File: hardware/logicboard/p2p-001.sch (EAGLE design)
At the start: 28 parts, among them IC11 74ALS04N, J0 DC9V, J11 AUDIO_JACK_3.5MM_PTH, J12 AUDIO_JACK_3.5MM_PTH, J13 AUDIO_JACK_3.5MM_PTH, J14 AUDIO_JACK_3.5MM_PTH, J7 DIN5, J8 DIN5, J9 DIN5, X0 MKDSN1,5/2-5,08

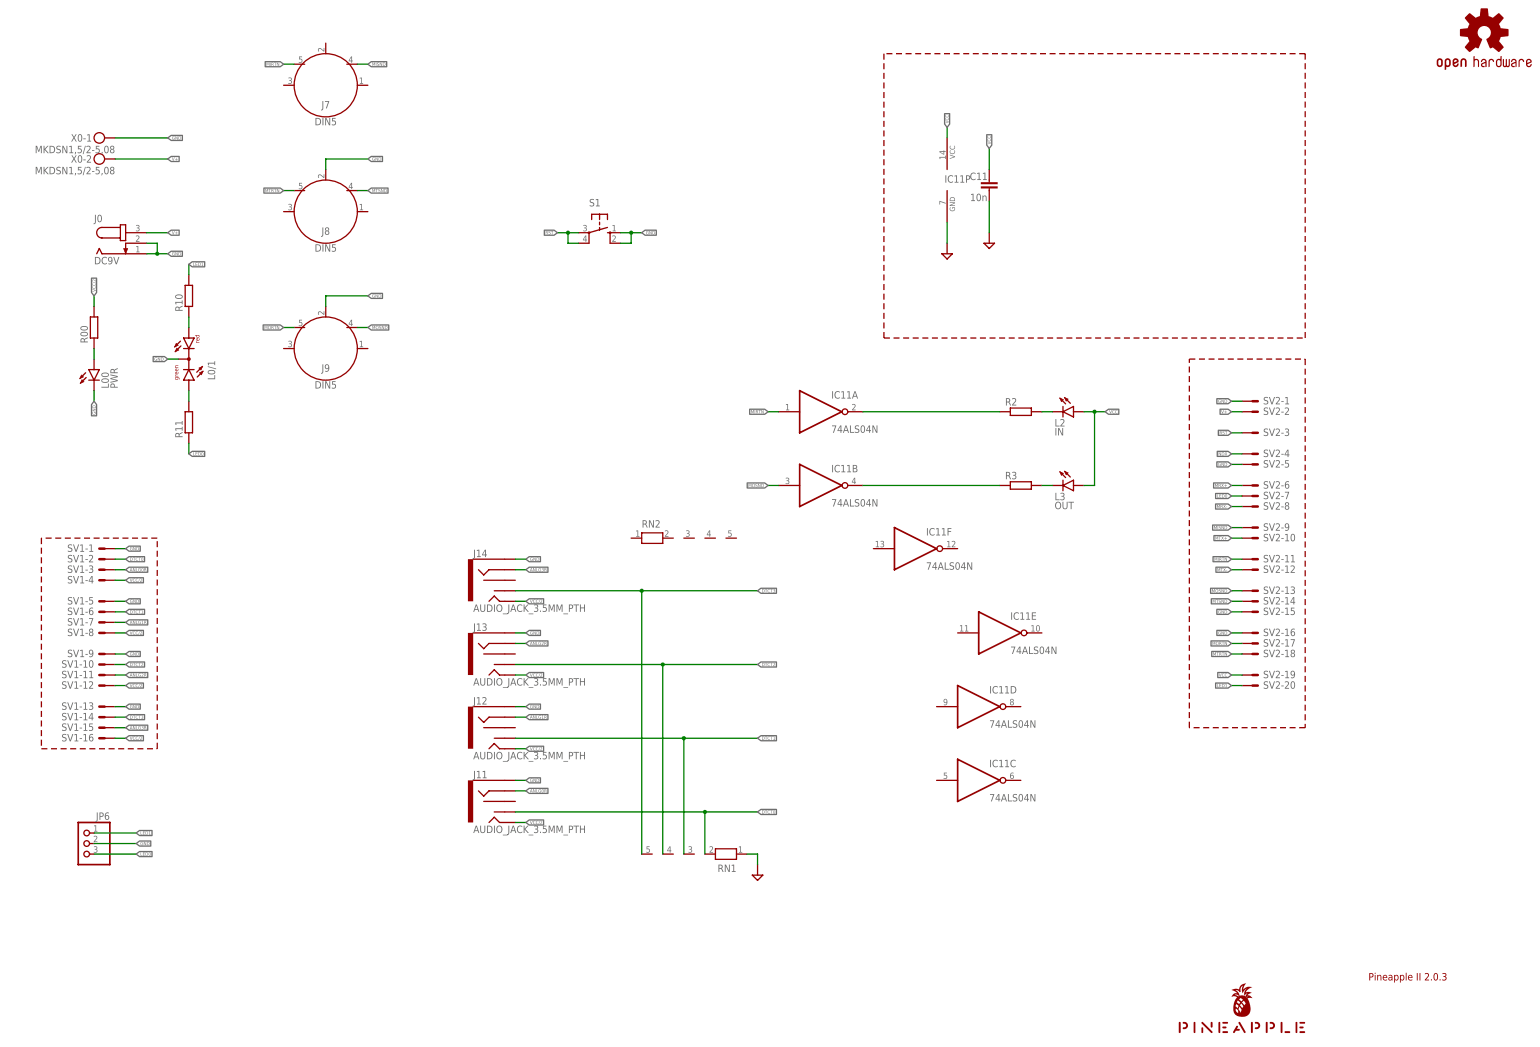
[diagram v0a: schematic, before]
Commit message: Cloud work...
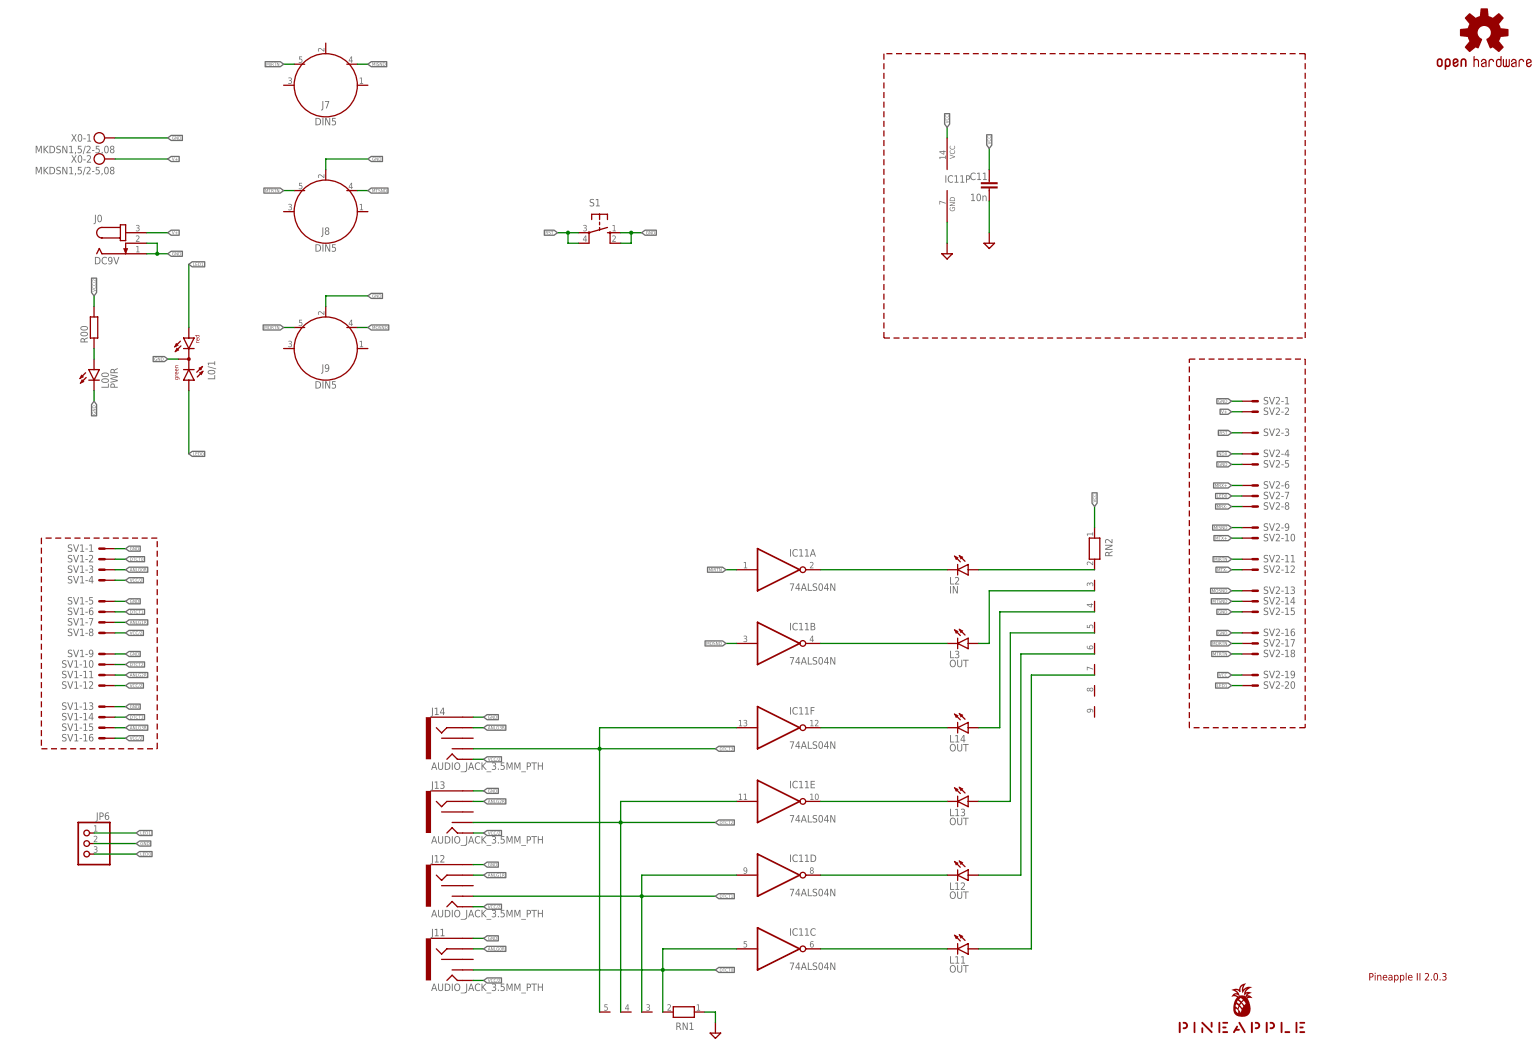
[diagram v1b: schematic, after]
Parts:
- removed R10, R11, R2, R3: (no value), rcl:R-EU_0204/5
- added L11, L12, L13, L14: OUT, led:LED3MM
- RN2: device resistor-net:RN04 -> resistor-net:RN08
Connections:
- removed net LED0A: L0/1.AG, R11.2
- removed net LED1A: L0/1.AR, R10.1
- removed net LEDMI: L2.C, R2.2
- removed net LEDMO: L3.C, R3.2
- new net N$10: IC11C.O, L11.C
- new net N$12: L12.A, RN2.6
- new net N$13: L11.A, RN2.7
- new net N$3: L2.A, RN2.2
- new net N$4: L3.A, RN2.3
- new net N$5: L14.A, RN2.4
- new net N$6: L13.A, RN2.5
- new net N$7: IC11F.O, L14.C
- new net N$8: IC11E.O, L13.C
- new net N$9: IC11D.O, L12.C
- net DTCT0: now also IC11C.I
- net DTCT1: now also IC11D.I
- net DTCT2: now also IC11E.I
- net DTCT3: now also IC11F.I
- net LED0: now also L0/1.AG; no longer R11.1
- net LED1: now also L0/1.AR; no longer R10.2
- net N$1: now also L2.C; no longer R2.1
- net N$2: now also L3.C; no longer R3.1
- net VCC: now also RN2.1; no longer L2.A, L3.A
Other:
- moved on the sheet: IC11A, IC11B, IC11C, IC11D, IC11E, IC11F, J11, J12, J13, J14, L2, L3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
